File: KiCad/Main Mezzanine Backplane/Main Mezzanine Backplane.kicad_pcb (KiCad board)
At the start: 4 copper layers, 48 x 97 mm, 42 parts, among them J1 BB0500220F-1002C-001, J2 BB0500220F-1002C-001, J3 FPC-05FB-50PH20, J4 FPC-05FB-50PH20, J5 FPC-05FB-50PH20, J6 FPC-05FB-50PH20, J7 FPC-05FB-50PH20, U1 D1213A-04S-7, U10 D1213A-04S-7, U11 D1213A-04S-7, U12 D1213A-04S-7, U13 D1213A-04S-7, U14 D1213A-04S-7, U15 D1213A-04S-7, U16 D1213A-04S-7, U17 D1213A-04S-7, U18 D1213A-04S-7, U19 D1213A-04S-7, U2 D1213A-04S-7, U20 D1213A-04S-7, U21 D1213A-04S-7, U22 D1213A-04S-7, U23 D1213A-04S-7, U24 D1213A-04S-7, U25 D1213A-04S-7, U26 D1213A-04S-7, U3 D1213A-04S-7, U4 D1213A-04S-7, U5 D1213A-04S-7, U6 D1213A-04S-7, U7 D1213A-04S-7, U8 D1213A-04S-7, U9 D1213A-04S-7

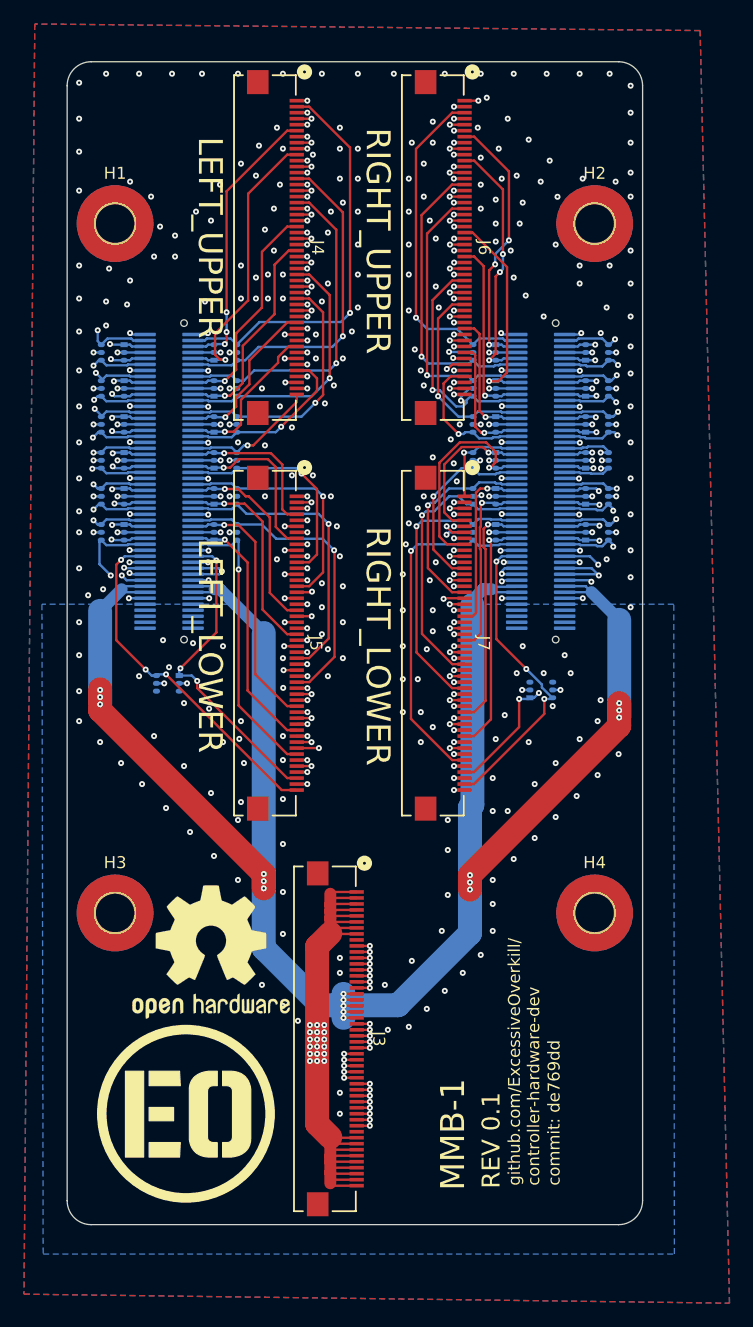
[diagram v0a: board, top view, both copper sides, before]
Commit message: update
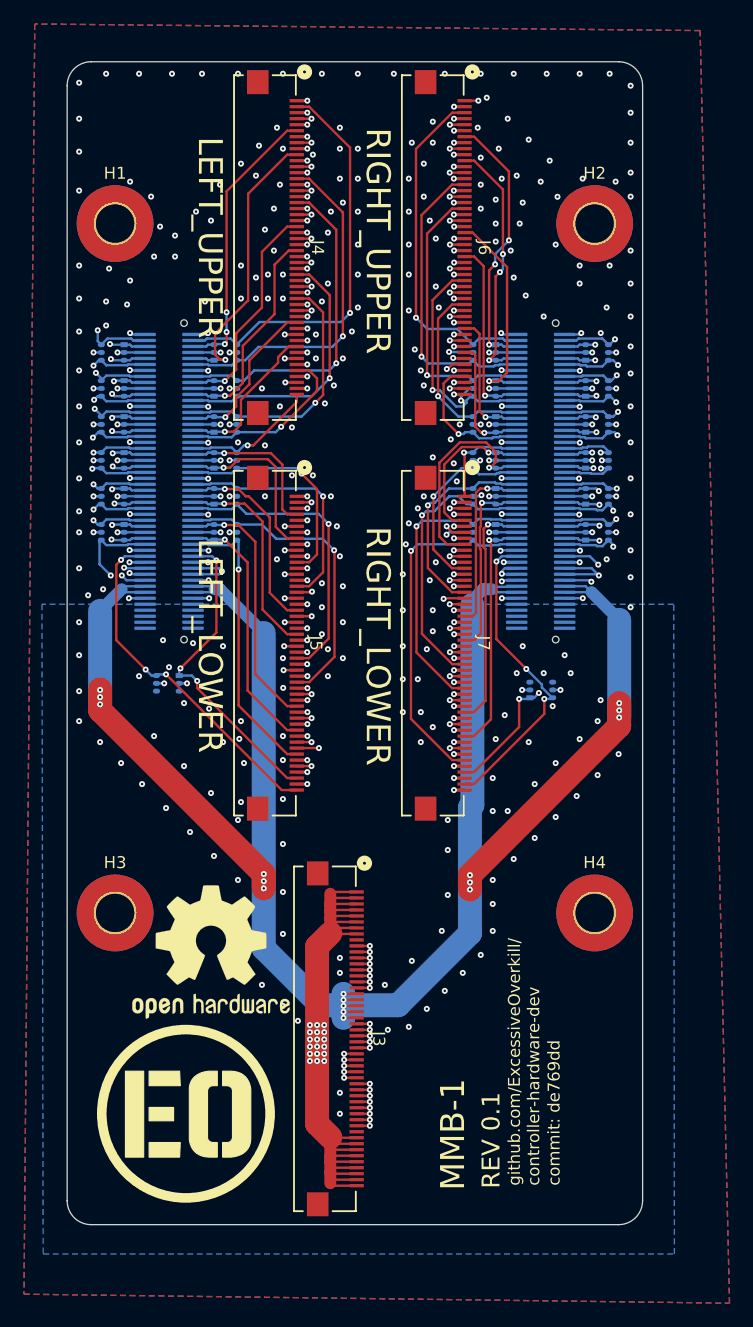
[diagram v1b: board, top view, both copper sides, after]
